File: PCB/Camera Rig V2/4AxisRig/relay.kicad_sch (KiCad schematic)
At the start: 5 parts, among them J2 SJ-3524-SMT, Q1 NMOS, Q2 NMOS

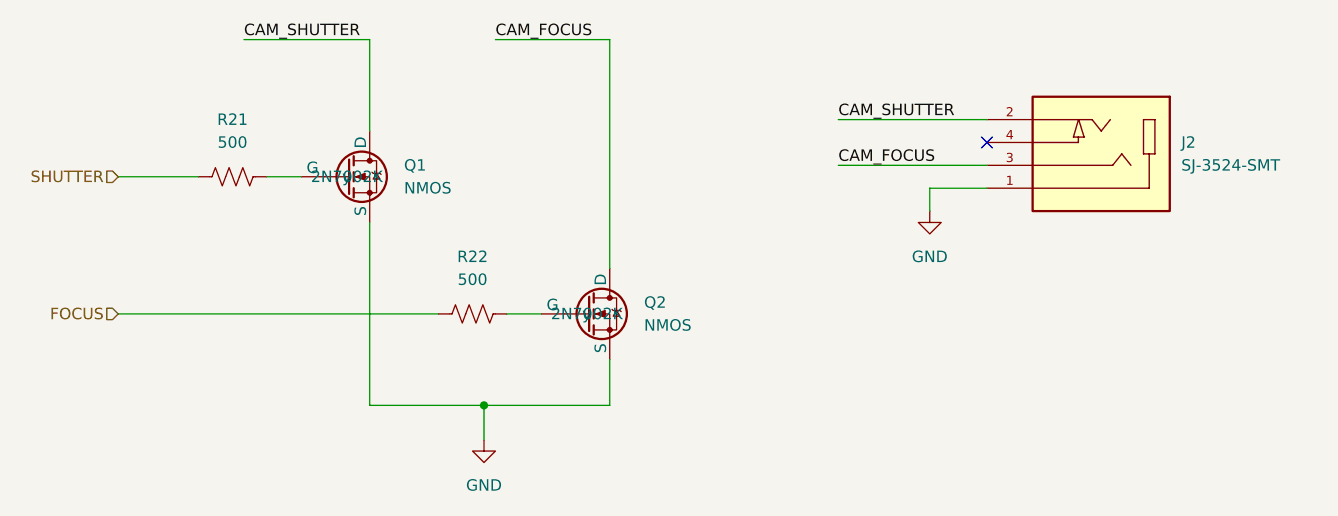
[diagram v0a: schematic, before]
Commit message: PCB V2 first draft
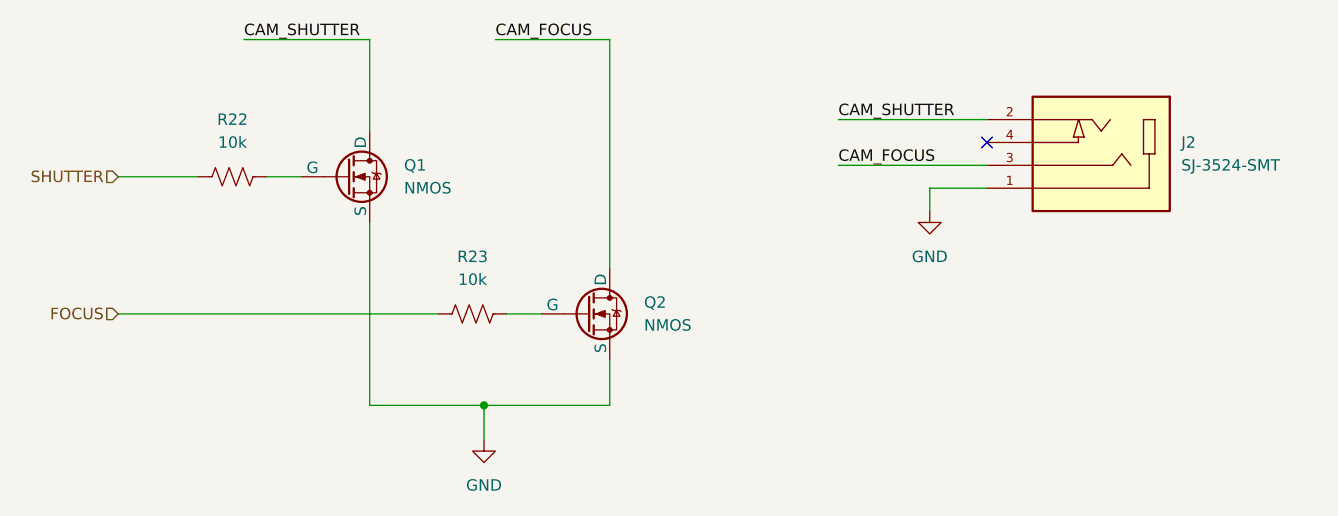
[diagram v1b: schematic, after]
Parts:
- Q1, Q2: Unique FP y -> (none)
- R22: renamed from R21; value 500 -> 10k
- R23: renamed from R22; value 500 -> 10k
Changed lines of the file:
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@@
 					(size 1.27 1.27)
 				)
-			)
-		)
-		(property "Unique FP" "y"
-			(at 140.97 107.95 0)
-			(effects
-				(font
-					(size 1.27 1.27)
-				)
+				(hide yes)
 			)
 		)
@@
 		(dnp no)
 		(fields_autoplaced yes)
-		(property "Reference" "R21"
+		(property "Reference" "R22"
 			(at 101.6 86.36 90)
 			(effects
@@
 			)
 		)
-		(property "Value" "500"
+		(property "Value" "10k"
 			(at 101.6 88.9 90)
 			(effects
@@
 			)
 		)
-		(property "Unique FP" ""
-			(at 101.6 92.71 0)
-			(effects
-				(font
-					(size 1.27 1.27)
-				)
-			)
-		)
 		(pin "1"
 		)
@@
 			(project ""
 				(path "/afe116b2-64d1-4090-9b3d-2b16ecf9512b/1f8c1e4e-252c-4fbf-9279-da2bb0a1e4d6"
-					(reference "R21")
+					(reference "R22")
 					(unit 1)
 				)
@@
 			)
 		)
-		(property "Unique FP" ""
-			(at 198.12 88.9 0)
-			(effects
-				(font
-					(size 1.27 1.27)
-				)
-			)
-		)
 		(pin "4"
 		)
@@
 		(dnp no)
 		(fields_autoplaced yes)
-		(property "Reference" "#PWR092"
+		(property "Reference" "#PWR049"
 			(at 179.07 102.87 0)
 			(effects
@@
 			(project "4AxisRig"
 				(path "/afe116b2-64d1-4090-9b3d-2b16ecf9512b/1f8c1e4e-252c-4fbf-9279-da2bb0a1e4d6"
-					(reference "#PWR092")
+					(reference "#PWR049")
 					(unit 1)
 				)
@@
 					(size 1.27 1.27)
 				)
-			)
-		)
-		(property "Unique FP" "y"
-			(at 114.3 92.71 0)
-			(effects
-				(font
-					(size 1.27 1.27)
-				)
+				(hide yes)
 			)
 		)
@@
 		(dnp no)
 		(fields_autoplaced yes)
-		(property "Reference" "#PWR047"
+		(property "Reference" "#PWR048"
 			(at 129.54 128.27 0)
 			(effects
@@
 			(project ""
 				(path "/afe116b2-64d1-4090-9b3d-2b16ecf9512b/1f8c1e4e-252c-4fbf-9279-da2bb0a1e4d6"
-					(reference "#PWR047")
+					(reference "#PWR048")
 					(unit 1)
 				)
@@
 		(dnp no)
 		(fields_autoplaced yes)
-		(property "Reference" "R22"
+		(property "Reference" "R23"
 			(at 128.27 101.6 90)
 			(effects
@@
 			)
 		)
-		(property "Value" "500"
+		(property "Value" "10k"
 			(at 128.27 104.14 90)
 			(effects
@@
 			)
 		)
-		(property "Unique FP" ""
-			(at 128.27 107.95 0)
-			(effects
-				(font
-					(size 1.27 1.27)
-				)
-			)
-		)
 		(pin "1"
 		)
@@
 			(project "4AxisRig"
 				(path "/afe116b2-64d1-4090-9b3d-2b16ecf9512b/1f8c1e4e-252c-4fbf-9279-da2bb0a1e4d6"
-					(reference "R22")
-					(unit 1)
-				)
+					(reference "R23")
+					(unit 1)
+				)
